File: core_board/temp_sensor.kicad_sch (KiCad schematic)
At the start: 3 parts

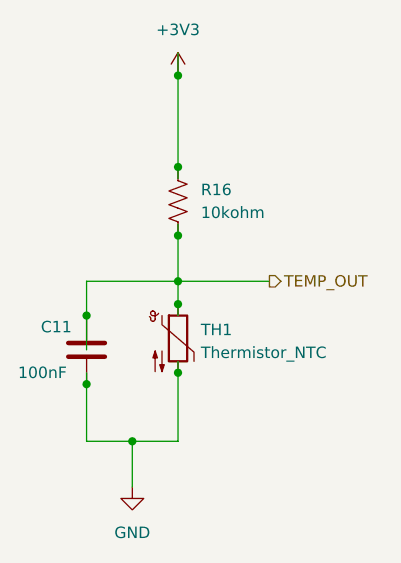
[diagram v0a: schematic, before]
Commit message: Finish Schematic
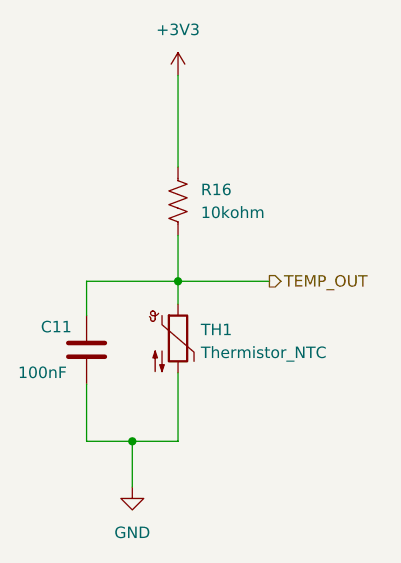
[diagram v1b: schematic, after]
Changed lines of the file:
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@@
 	(paper "A4")
-	(junction
-		(at 139.7 81.28)
-		(diameter 0)
-		(color 0 0 0 0)
-	)
-	(junction
-		(at 129.54 97.79)
-		(diameter 0)
-		(color 0 0 0 0)
-	)
 	(junction
 		(at 134.62 111.76)
@@
 	)
 	(junction
-		(at 139.7 96.52)
-		(diameter 0)
-		(color 0 0 0 0)
-	)
-	(junction
 		(at 139.7 93.98)
-		(diameter 0)
-		(color 0 0 0 0)
-	)
-	(junction
-		(at 139.7 104.14)
-		(diameter 0)
-		(color 0 0 0 0)
-	)
-	(junction
-		(at 139.7 88.9)
-		(diameter 0)
-		(color 0 0 0 0)
-	)
-	(junction
-		(at 139.7 71.12)
-		(diameter 0)
-		(color 0 0 0 0)
-	)
-	(junction
-		(at 129.54 105.41)
 		(diameter 0)
 		(color 0 0 0 0)
@@
 	(wire
 		(pts
-			(xy 129.54 93.98) (xy 129.54 101.6)
-		)
-		(stroke
-			(width 0)
-			(type default)
-		)
-	)
-	(wire
-		(pts
 			(xy 139.7 71.12) (xy 139.7 81.28)
-		)
-		(stroke
-			(width 0)
-			(type default)
-		)
-	)
-	(wire
-		(pts
-			(xy 139.7 96.52) (xy 139.7 97.79)
 		)
 		(stroke
@@
 	(wire
 		(pts
-			(xy 139.7 81.28) (xy 139.7 82.55)
-		)
-		(stroke
-			(width 0)
-			(type default)
-		)
-	)
-	(wire
-		(pts
-			(xy 129.54 104.14) (xy 129.54 105.41)
-		)
-		(stroke
-			(width 0)
-			(type default)
-		)
-	)
-	(wire
-		(pts
 			(xy 139.7 104.14) (xy 139.7 111.76)
-		)
-		(stroke
-			(width 0)
-			(type default)
-		)
-	)
-	(wire
-		(pts
-			(xy 139.7 87.63) (xy 139.7 88.9)
-		)
-		(stroke
-			(width 0)
-			(type default)
-		)
-	)
-	(wire
-		(pts
-			(xy 139.7 102.87) (xy 139.7 104.14)
 		)
 		(stroke
@@
 	(wire
 		(pts
-			(xy 139.7 68.58) (xy 139.7 71.12)
+			(xy 129.54 93.98) (xy 129.54 97.79)
 		)
 		(stroke
